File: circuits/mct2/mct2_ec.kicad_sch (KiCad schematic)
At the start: 1 part

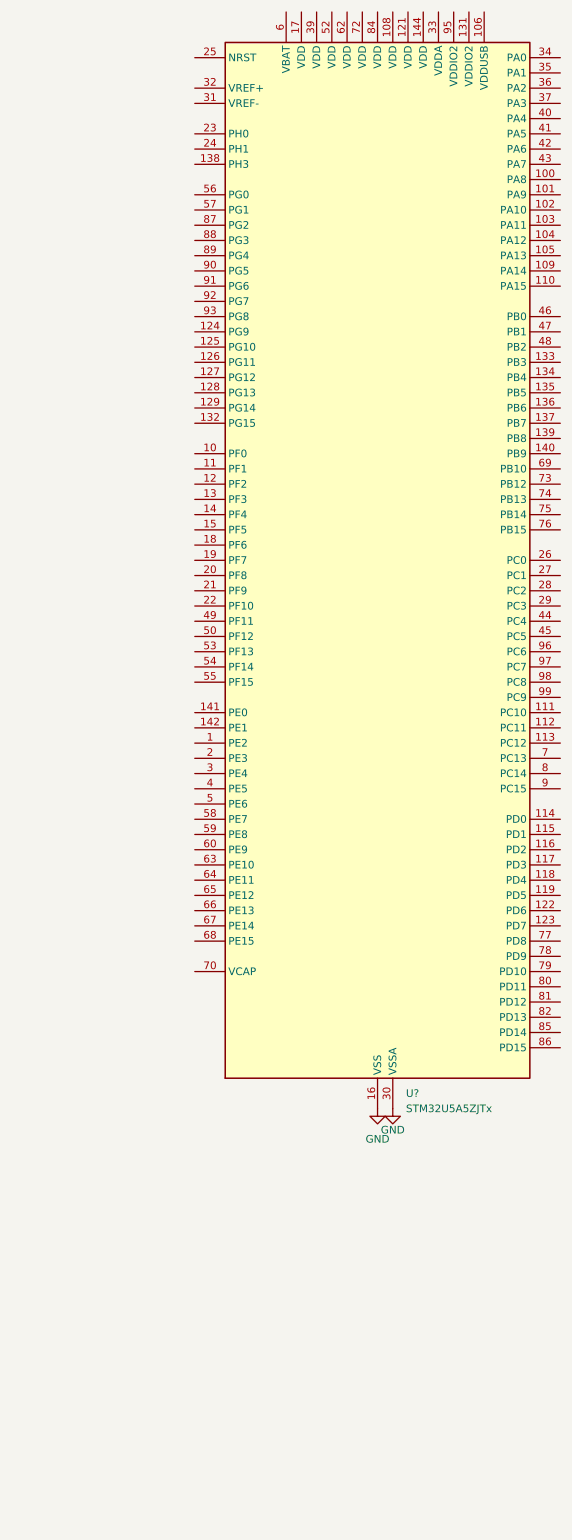
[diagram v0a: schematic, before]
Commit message: Aug 2, 2024
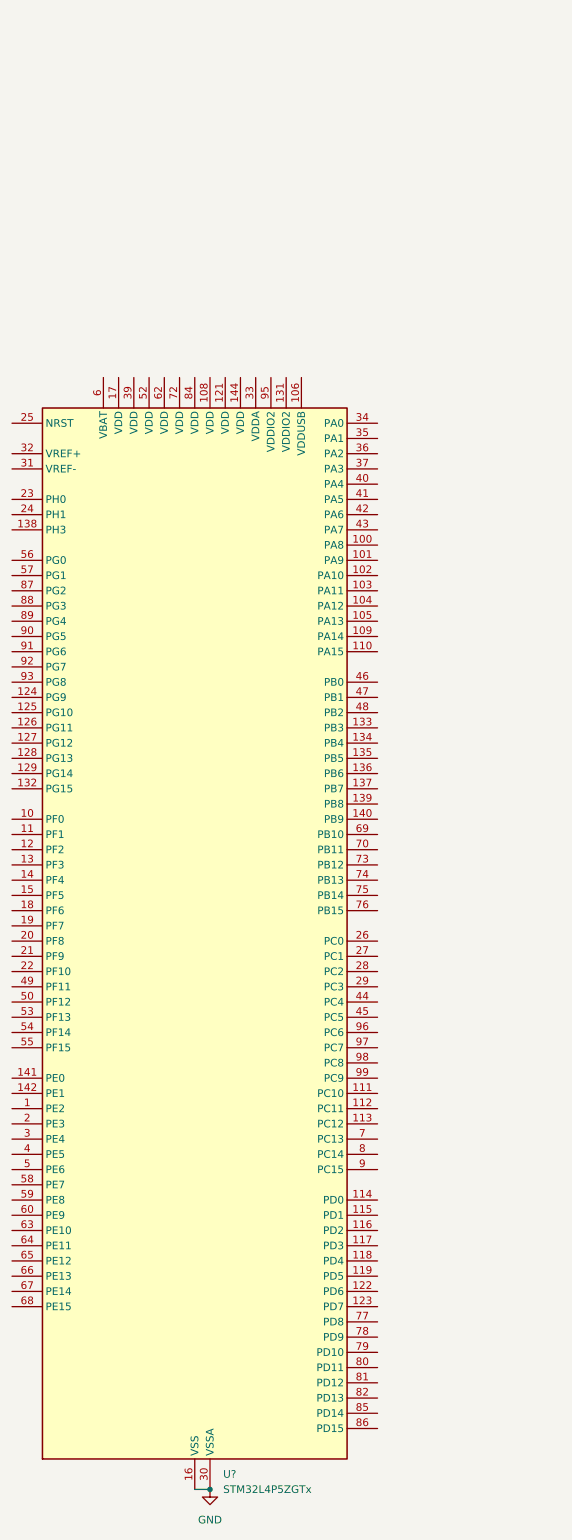
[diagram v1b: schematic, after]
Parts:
- removed U?: STM32U5A5ZJTx, Package_QFP:LQFP-144_20x20mm_P0.5mm, symbol MCU_ST_STM32U5:STM32U5A5ZJTx
- added U?: STM32L4P5ZGTx, Package_QFP:LQFP-144_20x20mm_P0.5mm, symbol MCU_ST_STM32L4:STM32L4P5ZGTx
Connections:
- net GND: now also U?.107 (VSS), U?.120 (VSS), U?.130 (VSS), U?.143 (VSS), U?.16 (VSS), U?.30 (VSSA), U?.38 (VSS), U?.51 (VSS), U?.61 (VSS), U?.71 (VSS), U?.83 (VSS), U?.94 (VSS)
